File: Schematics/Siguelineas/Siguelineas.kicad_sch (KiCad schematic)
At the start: 25 parts, among them J1 Batt_Input, J11 SD_con, J2 FAN_IN, J3 Line_Sensors, J3 TB6612FNG_A, J4 IMU, J4 TB6612FNG_B, J5 SCREEN, J8 Motor_1, J9 Motor_2, Q1 IRLML2502, Q2 IRLML2502, Q3 IRLML2502, SW1 Switch, SW2 Button 1, SW3 Button 2, U1 Mini360, U2 ESP32-DEVKIT-V1

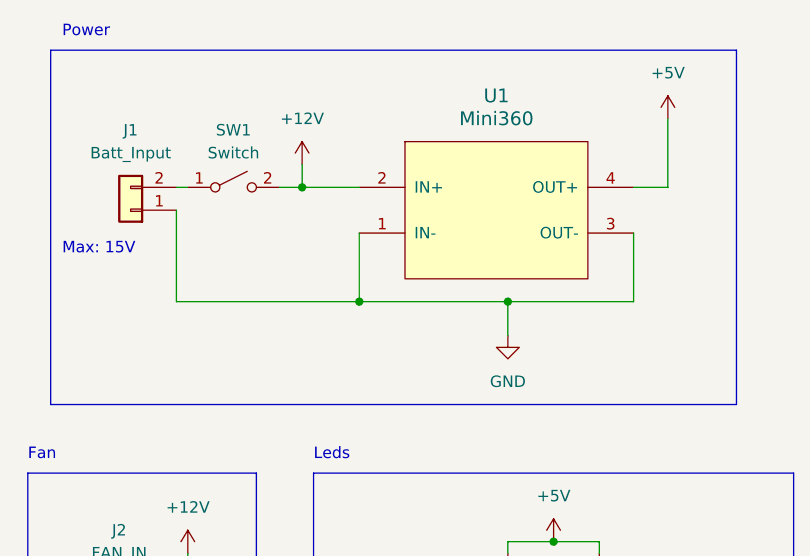
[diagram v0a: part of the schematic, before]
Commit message: Version 1.0
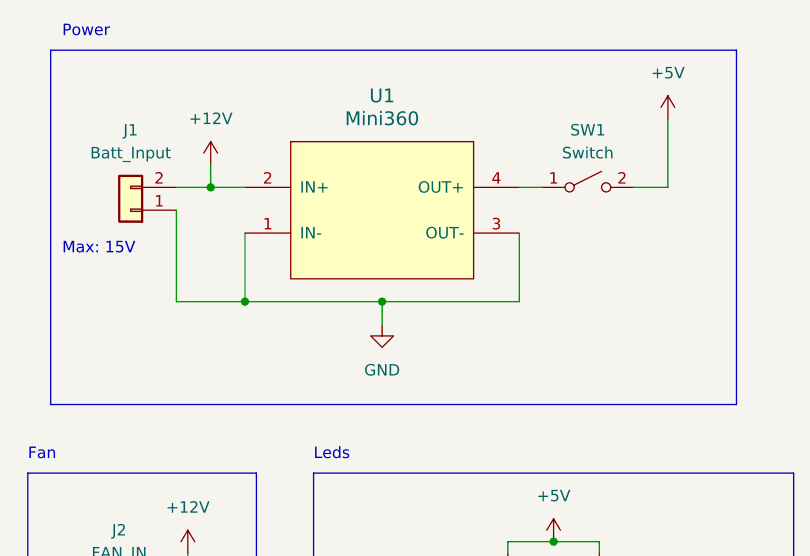
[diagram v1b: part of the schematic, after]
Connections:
- net +12V: now also J1.2 (Pin_2); no longer SW1.2 (B)
- net +5V: now also SW1.2 (B); no longer U1.4 (OUT+)
- net at SW1.1 (A): now also U1.4 (OUT+); no longer J1.2 (Pin_2)
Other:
- moved on the sheet: SW1, U1
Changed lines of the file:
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@@
     (comment 1 "Adrian Martinez")
   )
+  (junction (at 44.45 36.83) (diameter 0) (color 0 0 0 0)
+  )
   (junction (at 82.55 107.95) (diameter 0) (color 0 0 0 0)
   )
-  (junction (at 54.61 36.83) (diameter 0) (color 0 0 0 0)
-  )
   (junction (at 256.54 138.43) (diameter 0) (color 0 0 0 0)
   )
@@
   (junction (at 143.51 139.7) (diameter 0) (color 0 0 0 0)
   )
-  (junction (at 60.96 49.53) (diameter 0) (color 0 0 0 0)
+  (junction (at 63.5 49.53) (diameter 0) (color 0 0 0 0)
   )
   (junction (at 259.08 125.73) (diameter 0) (color 0 0 0 0)
@@
   (junction (at 256.54 148.59) (diameter 0) (color 0 0 0 0)
   )
-  (junction (at 77.47 49.53) (diameter 0) (color 0 0 0 0)
-  )
   (junction (at 256.54 140.97) (diameter 0) (color 0 0 0 0)
   )
   (junction (at 43.18 168.91) (diameter 0) (color 0 0 0 0)
+  )
+  (junction (at 48.26 49.53) (diameter 0) (color 0 0 0 0)
   )
   (junction (at 143.51 163.83) (diameter 0) (color 0 0 0 0)
@@
   (no_connect (at 262.89 143.51))
   (no_connect (at 262.89 146.05))
-  (wire (pts (xy 52.07 36.83) (xy 54.61 36.83))
-    (stroke (width 0) (type default))
-  )
   (wire (pts (xy 40.64 161.29) (xy 49.53 161.29))
     (stroke (width 0) (type default))
@@
     (stroke (width 0) (type default))
   )
+  (wire (pts (xy 63.5 49.53) (xy 78.74 49.53))
+    (stroke (width 0) (type default))
+  )
   (wire (pts (xy 40.64 158.75) (xy 49.53 158.75))
     (stroke (width 0) (type default))
@@
     (stroke (width 0) (type default))
   )
-  (wire (pts (xy 54.61 36.83) (xy 54.61 34.29))
+  (wire (pts (xy 44.45 36.83) (xy 44.45 34.29))
     (stroke (width 0) (type default))
   )
@@
     (stroke (width 0) (type default))
   )
+  (wire (pts (xy 44.45 36.83) (xy 48.26 36.83))
+    (stroke (width 0) (type default))
+  )
   (wire (pts (xy 87.63 95.25) (xy 87.63 97.79))
     (stroke (width 0) (type default))
@@
     (stroke (width 0) (type default))
   )
-  (wire (pts (xy 60.96 41.91) (xy 60.96 49.53))
+  (wire (pts (xy 48.26 41.91) (xy 48.26 49.53))
     (stroke (width 0) (type default))
   )
@@
     (stroke (width 0) (type default))
   )
+  (wire (pts (xy 91.44 36.83) (xy 95.25 36.83))
+    (stroke (width 0) (type default))
+  )
   (wire (pts (xy 256.54 138.43) (xy 262.89 138.43))
     (stroke (width 0) (type default))
@@
     (stroke (width 0) (type default))
   )
+  (wire (pts (xy 48.26 49.53) (xy 63.5 49.53))
+    (stroke (width 0) (type default))
+  )
   (wire (pts (xy 237.49 39.37) (xy 228.6 39.37))
     (stroke (width 0) (type default))
@@
     (stroke (width 0) (type default))
   )
-  (wire (pts (xy 91.44 36.83) (xy 95.25 36.83))
-    (stroke (width 0) (type default))
-  )
   (wire (pts (xy 39.37 83.82) (xy 41.91 83.82))
     (stroke (width 0) (type default))
@@
     (stroke (width 0) (type default))
   )
+  (wire (pts (xy 78.74 36.83) (xy 81.28 36.83))
+    (stroke (width 0) (type default))
+  )
   (wire (pts (xy 41.91 77.47) (xy 41.91 81.28))
     (stroke (width 0) (type default))
@@
     (stroke (width 0) (type default))
   )
-  (wire (pts (xy 77.47 49.53) (xy 77.47 53.34))
+  (wire (pts (xy 63.5 49.53) (xy 63.5 52.07))
     (stroke (width 0) (type default))
   )
@@
     (stroke (width 0) (type default))
   )
-  (wire (pts (xy 54.61 36.83) (xy 60.96 36.83))
-    (stroke (width 0) (type default))
-  )
-  (wire (pts (xy 40.64 49.53) (xy 60.96 49.53))
+  (wire (pts (xy 40.64 49.53) (xy 48.26 49.53))
     (stroke (width 0) (type default))
   )
@@
     (stroke (width 0) (type default))
   )
-  (wire (pts (xy 40.64 36.83) (xy 41.91 36.83))
-    (stroke (width 0) (type default))
-  )
   (wire (pts (xy 76.2 153.67) (xy 69.85 153.67))
     (stroke (width 0) (type default))
@@
     (stroke (width 0) (type default))
   )
-  (wire (pts (xy 60.96 49.53) (xy 77.47 49.53))
-    (stroke (width 0) (type default))
-  )
   (wire (pts (xy 175.26 101.6) (xy 176.53 101.6))
     (stroke (width 0) (type default))
@@
     (stroke (width 0) (type default))
   )
-  (wire (pts (xy 91.44 49.53) (xy 77.47 49.53))
-    (stroke (width 0) (type default))
-  )
   (wire (pts (xy 49.53 166.37) (xy 40.64 166.37))
     (stroke (width 0) (type default))
   )
+  (wire (pts (xy 40.64 36.83) (xy 44.45 36.83))
+    (stroke (width 0) (type default))
+  )
   (wire (pts (xy 82.55 76.2) (xy 87.63 76.2))
     (stroke (width 0) (type default))
@@
     (stroke (width 0) (type default))
   )
-  (wire (pts (xy 91.44 41.91) (xy 91.44 49.53))
+  (wire (pts (xy 78.74 41.91) (xy 78.74 49.53))
     (stroke (width 0) (type default))
   )
@@
     )
   )
-  (symbol (lib_id "Switch:SW_SPST") (at 46.99 36.83 0) (unit 1)
-    (in_bom yes) (on_board yes) (dnp no) (fields_autoplaced)
-    (property "Reference" "SW1" (at 46.99 30.48 0)
-      (effects (font (size 1.27 1.27)))
-    )
-    (property "Value" "Switch" (at 46.99 33.02 0)
-      (effects (font (size 1.27 1.27)))
-    )
-    (property "Footprint" "Button_Switch_THT:SW_CuK_OS102011MA1QN1_SPDT_Angled" (at 46.99 36.83 0)
-      (effects (font (size 1.27 1.27)) hide)
-    )
-    (property "Datasheet" "~" (at 46.99 36.83 0)
+  (symbol (lib_id "Switch:SW_SPST") (at 86.36 36.83 0) (unit 1)
+    (in_bom yes) (on_board yes) (dnp no) (fields_autoplaced)
+    (property "Reference" "SW1" (at 86.36 30.48 0)
+      (effects (font (size 1.27 1.27)))
+    )
+    (property "Value" "Switch" (at 86.36 33.02 0)
+      (effects (font (size 1.27 1.27)))
+    )
+    (property "Footprint" "Button_Switch_THT:SW_CuK_OS102011MA1QN1_SPDT_Angled" (at 86.36 36.83 0)
+      (effects (font (size 1.27 1.27)) hide)
+    )
+    (property "Datasheet" "~" (at 86.36 36.83 0)
       (effects (font (size 1.27 1.27)) hide)
     )
@@
     )
   )
-  (symbol (lib_id "power:+12V") (at 54.61 34.29 0) (unit 1)
-    (in_bom yes) (on_board yes) (dnp no) (fields_autoplaced)
-    (property "Reference" "#PWR01" (at 54.61 38.1 0)
-      (effects (font (size 1.27 1.27)) hide)
-    )
-    (property "Value" "+12V" (at 54.61 29.21 0)
-      (effects (font (size 1.27 1.27)))
-    )
-    (property "Footprint" "" (at 54.61 34.29 0)
-      (effects (font (size 1.27 1.27)) hide)
-    )
-    (property "Datasheet" "" (at 54.61 34.29 0)
+  (symbol (lib_id "power:+12V") (at 44.45 34.29 0) (unit 1)
+    (in_bom yes) (on_board yes) (dnp no) (fields_autoplaced)
+    (property "Reference" "#PWR01" (at 44.45 38.1 0)
+      (effects (font (size 1.27 1.27)) hide)
+    )
+    (property "Value" "+12V" (at 44.45 29.21 0)
+      (effects (font (size 1.27 1.27)))
+    )
+    (property "Footprint" "" (at 44.45 34.29 0)
+      (effects (font (size 1.27 1.27)) hide)
+    )
+    (property "Datasheet" "" (at 44.45 34.29 0)
       (effects (font (size 1.27 1.27)) hide)
     )
@@
     )
   )
-  (symbol (lib_id "power:GND") (at 77.47 53.34 0) (unit 1)
+  (symbol (lib_id "power:GND") (at 63.5 52.07 0) (unit 1)
     (in_bom yes) (on_board yes) (dnp no)
-    (property "Reference" "#PWR02" (at 77.47 59.69 0)
-      (effects (font (size 1.27 1.27)) hide)
-    )
-    (property "Value" "GND" (at 77.47 58.42 0)
-      (effects (font (size 1.27 1.27)))
-    )
-    (property "Footprint" "" (at 77.47 53.34 0)
-      (effects (font (size 1.27 1.27)) hide)
-    )
-    (property "Datasheet" "" (at 77.47 53.34 0)
+    (property "Reference" "#PWR02" (at 63.5 58.42 0)
+      (effects (font (size 1.27 1.27)) hide)
+    )
+    (property "Value" "GND" (at 63.5 57.15 0)
+      (effects (font (size 1.27 1.27)))
+    )
+    (property "Footprint" "" (at 63.5 52.07 0)
+      (effects (font (size 1.27 1.27)) hide)
+    )
+    (property "Datasheet" "" (at 63.5 52.07 0)
       (effects (font (size 1.27 1.27)) hide)
     )
@@
     )
   )
-  (symbol (lib_id "mini360:Mini360") (at 76.2 39.37 0) (unit 1)
-    (in_bom yes) (on_board yes) (dnp no) (fields_autoplaced)
-    (property "Reference" "U1" (at 76.2 26.67 0)
+  (symbol (lib_id "mini360:Mini360") (at 63.5 39.37 0) (unit 1)
+    (in_bom yes) (on_board yes) (dnp no) (fields_autoplaced)
+    (property "Reference" "U1" (at 63.5 26.67 0)
       (effects (font (size 1.524 1.524)))
     )
-    (property "Value" "Mini360" (at 76.2 29.21 0)
+    (property "Value" "Mini360" (at 63.5 29.21 0)
       (effects (font (size 1.524 1.524)))
     )
-    (property "Footprint" "Mini360_step-down:Mini360_step-down" (at 76.2 39.37 0)
+    (property "Footprint" "Mini360_step-down:Mini360_step-down" (at 63.5 39.37 0)
       (effects (font (size 1.524 1.524)) hide)
     )
-    (property "Datasheet" "" (at 76.2 39.37 0)
+    (property "Datasheet" "" (at 63.5 39.37 0)
       (effects (font (size 1.524 1.524)) hide)
     )
